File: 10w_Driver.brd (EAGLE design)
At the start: 47 x 47 mm, 35 parts, among them IC1 78L05Z, IC2 WS2811-SOP8, T1 2N3904, T2 2N3904, T3 2N3904, U1 PT4115PT4115B89E, U2 PT4115PT4115B89E, U3 PT4115PT4115B89E, X1 22-23-2031, X2 22-23-2031, X3 LED-PAD, X4 LED-PAD, X5 LED-PAD, X6 LED-PAD, X7 LED-PAD, X8 LED-PAD

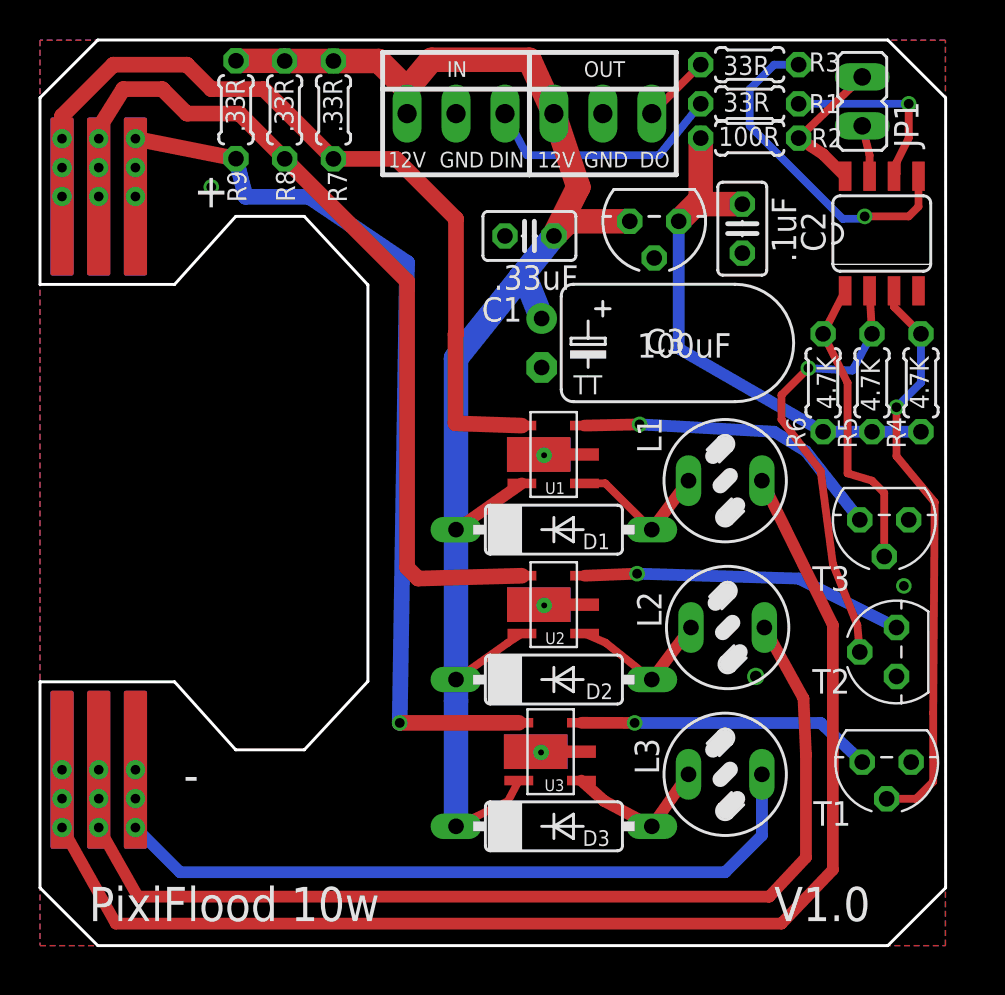
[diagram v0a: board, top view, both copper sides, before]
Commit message: Final 1.1
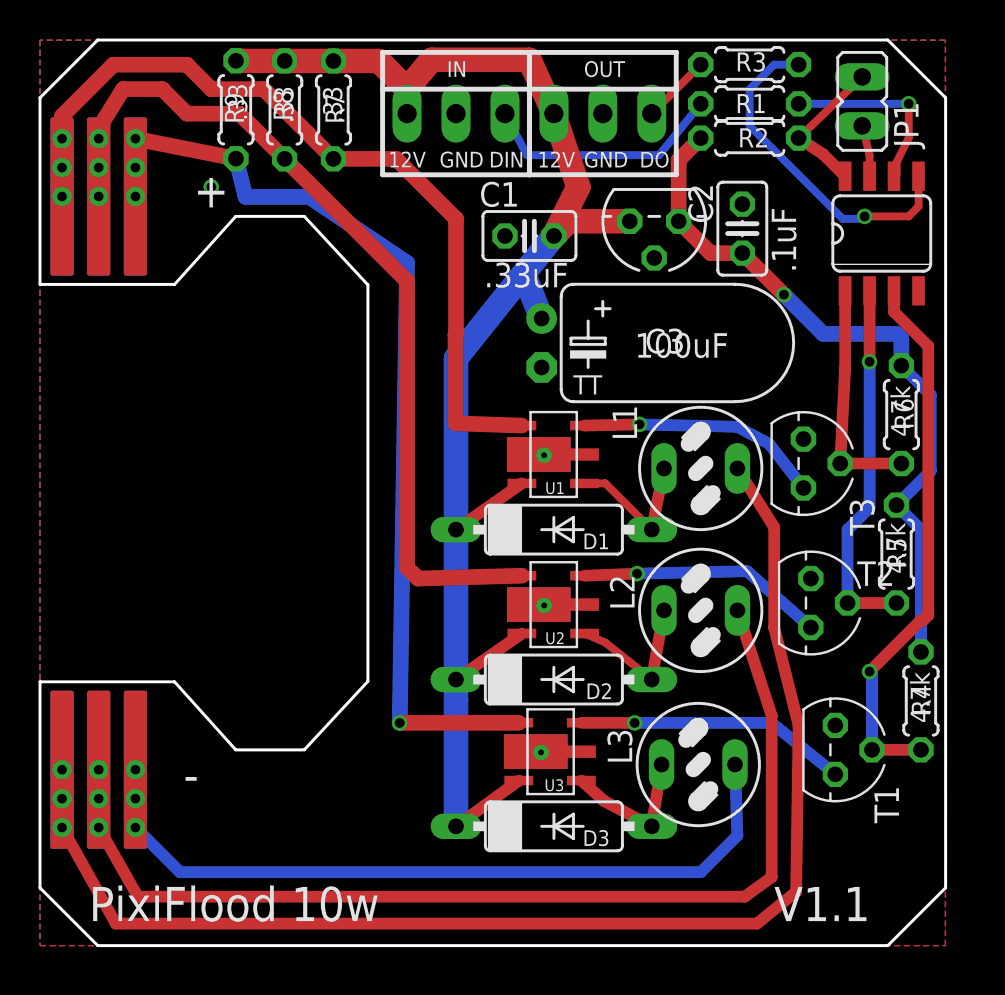
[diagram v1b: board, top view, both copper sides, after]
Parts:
- R2: value 100R -> 100ohm
- R4, R5, R6: value 4.7K -> 4.7k
- R7, R8, R9: value .33R -> .33
- moved R4 16.5 mm to (45.7, 12.7), turned to 270 degrees
- moved R5 8.98 mm to (44.5, 20.3), turned to 270 degrees
- moved T2 5.12 mm to (40.0, 17.8), turned to 270 degrees
- moved T3 5.11 mm to (39.6, 25.0), turned to 270 degrees
- moved R6 4.39 mm to (44.7, 27.6), turned to 270 degrees
- moved T1 2.74 mm to (41.3, 10.2), turned to 270 degrees
- moved L2 1.66 mm to (34.3, 17.4)
- moved L3 1.49 mm to (34.2, 9.40)
- moved L1 1.42 mm to (34.3, 24.8)
- turned C2 to 90 degrees
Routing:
- net +5V: track 27.4 -> 37.0 mm, vias 0 -> 1
- net GREEN: track 16.8 -> 12.9 mm
- net N$18: track 23.0 -> 19.2 mm
- net RED: track 16.3 -> 12.7 mm
- net N$20: track 15.6 -> 12.1 mm
- net N$15: track 30.1 -> 28.5 mm
- net BLUE: track 15.4 -> 14.1 mm
- net N$3: track 68.2 -> 67.3 mm
- net N$10: track 37.4 -> 36.7 mm
- net N$9: track 55.1 -> 54.5 mm
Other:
- board text added: "V1.1"
- board text removed: "V1.0"

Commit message: Final 1.1 with Inverter
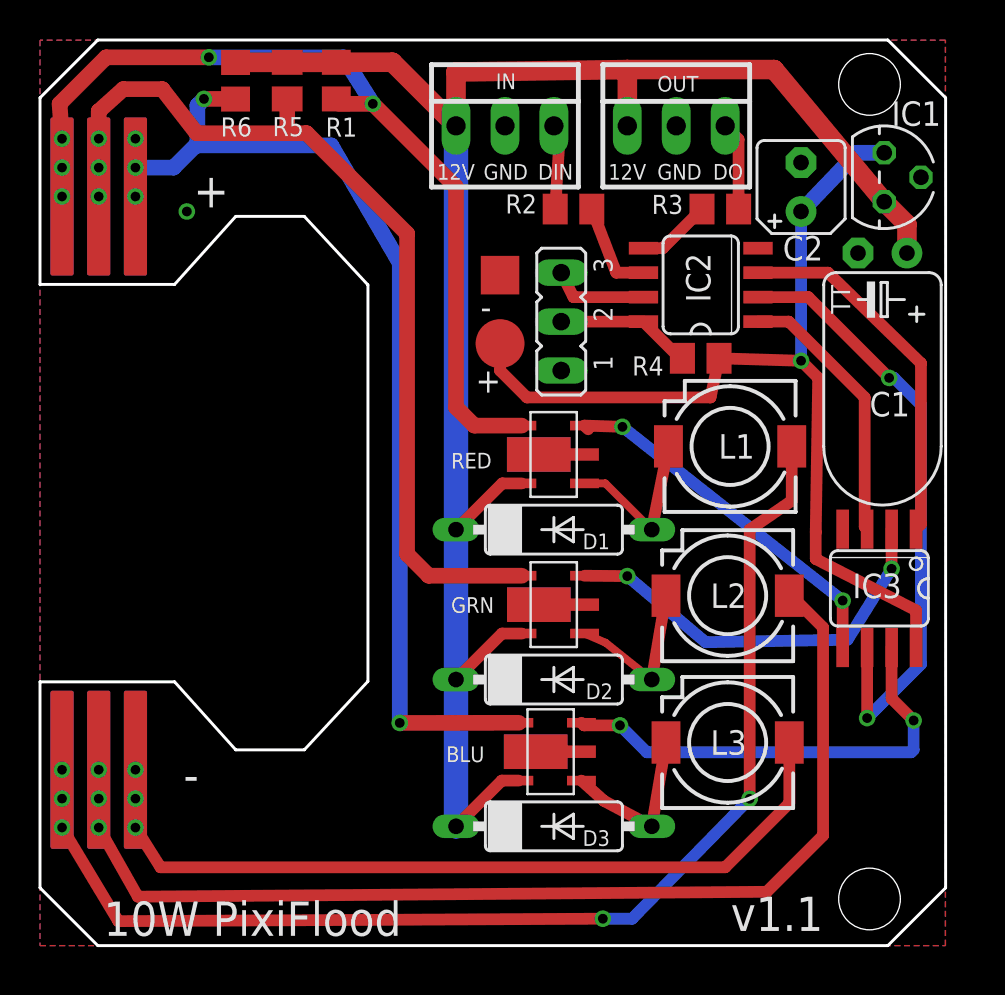
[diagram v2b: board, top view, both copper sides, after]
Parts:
- removed C3: 100uF, rcl:TT2D6L
- removed R7, R8, R9: .33, resistor:0204/5
- removed T1, T2, T3: 2N3904, transistor:TO92
- added IC3: TC7W04FTC7W04F, MyLibrary:SO08
- added TP1: TPB2,54, testpad:B2,54
- added TP2: PTR1TP20SQ, testpad:TP20SQ
- C1: value .33uF -> EL 100uF; device rcl:C025-025X050 -> rcl:TT2D6L
- C2: device rcl:C025-025X050 -> resistor:B45181A
- JP1: device jumper:JP1 -> jumper:JP2
- L1, L2, L3: value 82114R -> SLF7045; device inductors:82114R -> inductors:SLF7045
- R1: value 33R -> .3ohm .25w; device rcl:0204/5 -> resistor:R0805
- R2: value 100ohm -> 33R; device rcl:0204/5 -> rcl:M0805
- R3: device rcl:0204/5 -> rcl:M0805
- R4: value 4.7k -> 100ohm; device resistor:0204/5 -> rcl:M0805
- R5: value 4.7k -> .3hm .25w; device resistor:0204/5 -> resistor:M0805
- R6: value 4.7k -> .3ohm .25w; device resistor:0204/5 -> resistor:R0805
- U1, U2, U3: device MyLibrary:SOT89-5 -> IC:SOT89-5
- X2: value 22-23-2031 -> LED-PAD; device MyLibrary:22-23-2031 -> MyLibrary:LED-PAD
- X4: value LED-PAD -> 22-23-2031; device MyLibrary:LED-PAD -> MyLibrary:22-23-2031
- moved X4 47.3 mm to (33.0, 42.5), turned to 0 degrees
- moved R5 40.0 mm to (12.8, 44.9), turned to 90 degrees
- moved R6 38.7 mm to (10.1, 44.9), turned to 90 degrees
- moved X3 32.8 mm to (1.14, 7.62), turned to 180 degrees
- moved X2 28.2 mm to (1.14, 40.4)
- moved R1 21.5 mm to (15.4, 44.9), turned to 90 degrees
- moved R4 21.1 mm to (34.3, 30.5), turned to 180 degrees
- moved JP1 19.4 mm to (27.1, 32.4), turned to 90 degrees
- moved C1 18.3 mm to (43.7, 35.9)
- moved IC1 12.2 mm to (43.8, 39.9), turned to 270 degrees
- moved R2 9.86 mm to (27.7, 38.2)
- moved IC2 9.77 mm to (34.3, 34.3), turned to 90 degrees
- moved R3 7.65 mm to (35.3, 38.2), turned to 180 degrees
- moved C2 3.74 mm to (39.5, 39.4)
- moved X1 2.62 mm to (24.1, 42.5)
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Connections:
- removed net N$20: IC2.1, R6.2, T3.2
- new net N$19: IC2.2, IC3.6
- net +12V: now also C1.+, R1.2, R5.2, R6.2, X4.1; no longer C1.1, C3.+, R7.1, R8.1, R9.1, X2.1
- net +5V: now also C2.+, IC3.8, TP1.TP; no longer C2.1, R2.1, R5.1, R6.1
- net BLUE: now also IC3.7; no longer T1.1
- net BOUT: now also R6.1; no longer R9.2
- net GND: now also C1.-, C2.-, IC3.4, TP2.TP, X4.2; no longer C1.2, C2.2, C3.-, T1.3, T2.3, T3.3, U1.2A@1, U1.2A@2, U2.2A@1, U2.2A@2, U3.2A@1, U3.2A@2, X2.2
- net GOUT: now also R5.1; no longer R8.2
- net GREEN: now also IC3.2; no longer T2.1
- net N$14: now also JP1.2, R4.2; no longer JP1.1, R2.2
- net N$15: now also IC2.1, IC3.3; no longer IC2.3, R4.2, T1.2
- net N$16: now also IC2.3, IC3.1; no longer IC2.7, JP1.2
- net N$18: now also IC2.7, JP1.3; no longer IC2.2, R5.2, T2.2
- net N$3: now also X3.P$1@1, X3.P$1@2, X3.P$1@3; no longer X4.P$1@1, X4.P$1@2, X4.P$1@3
- net N$4: now also X4.3; no longer X2.3
- net N$6: now also R2.1; no longer R1.1
- net N$8: now also R2.2; no longer R1.2
- net RED: now also IC3.5; no longer T3.1
- net ROUT: now also R1.1, X2.P$1@1, X2.P$1@2, X2.P$1@3; no longer R7.2, X3.P$1@1, X3.P$1@2, X3.P$1@3
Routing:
- net N$19: track 0.00 -> 31.8 mm, vias 0 -> 2
- net +12V: track 79.3 -> 96.5 mm
- net N$16: track 2.66 -> 19.1 mm
- net N$15: track 28.5 -> 14.1 mm, vias 1 -> 0
- net N$18: track 19.2 -> 5.05 mm, vias 1 -> 0
- net +5V: track 37.0 -> 51.0 mm
- net N$7: track 17.6 -> 3.88 mm, vias 1 -> 0
- net N$20: track 12.1 -> 0.00 mm
- net BLUE: track 14.1 -> 23.7 mm, vias 1 -> 2
- net GREEN: track 12.9 -> 21.3 mm, vias 1 -> 2
- net N$6: track 12.7 -> 4.46 mm
- net RED: track 12.7 -> 19.2 mm, vias 1 -> 2
- net N$10: track 36.7 -> 42.6 mm
- net BOUT: track 49.9 -> 55.1 mm, vias 1 -> 2
- net N$8: track 9.68 -> 4.95 mm, vias 1 -> 0
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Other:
- board text added: "10W PixiFlood"
- board text added: "AJ Reynolds"
- board text added: "BLU"
- board text added: "GRN"
- board text added: "RED"
- board text added: "v1.1"
- board text removed: "PixiFlood 10w"
- board text removed: "V1.1"
